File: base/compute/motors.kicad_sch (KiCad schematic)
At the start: 17 parts, among them U4 W25X20CLSN, U5 ICE40UP5K-SG48ITR-FPGA_Lattice

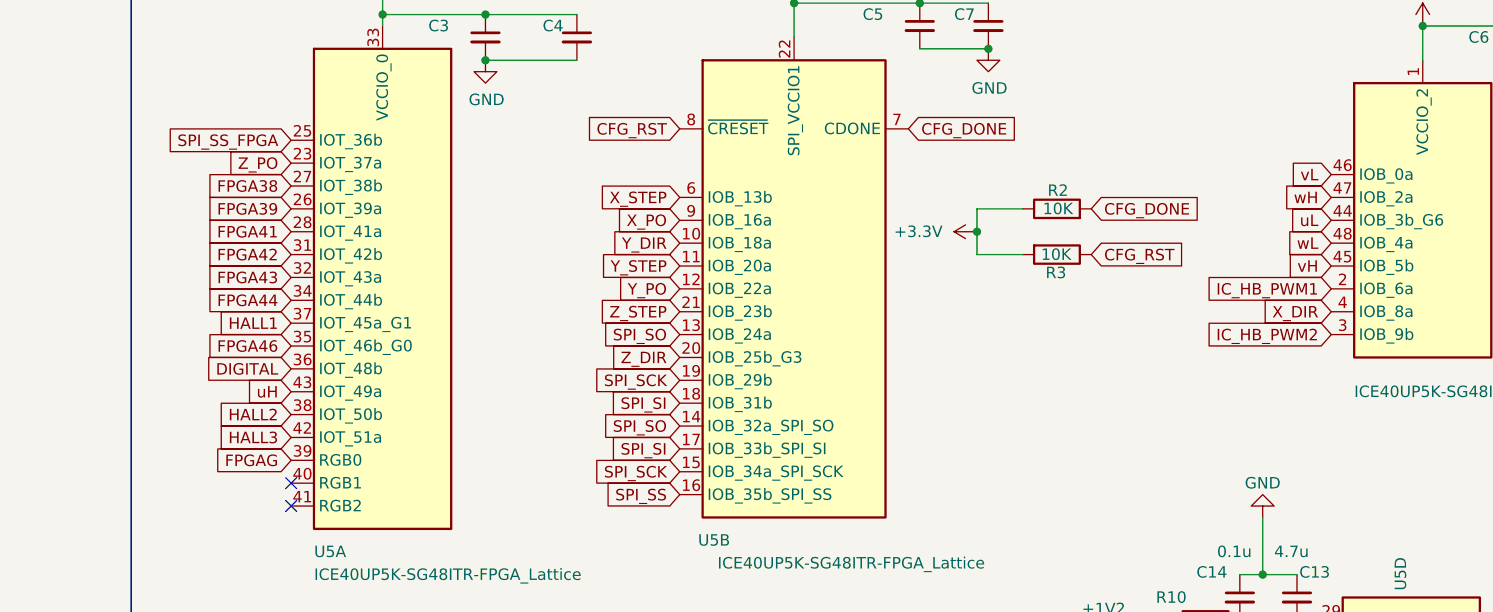
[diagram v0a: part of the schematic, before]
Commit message: retracking board
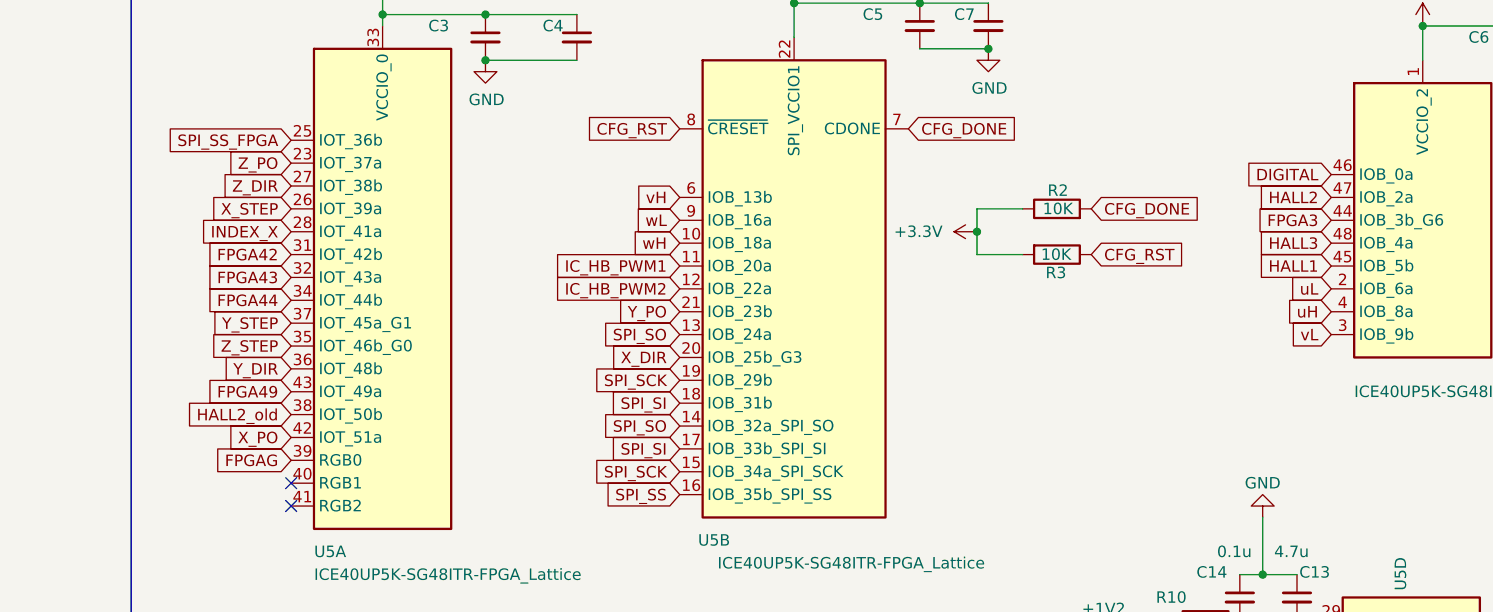
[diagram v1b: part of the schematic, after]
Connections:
- net FPGA38 is gone; now on net Z_DIR: U5.27 (IOT_38b)
- net FPGA39 is gone; now on net X_STEP: U5.26 (IOT_39a)
- net FPGA46 is gone; now on net Z_STEP: U5.35 (IOT_46b_G0)
- net DIGITAL: now also U5.46 (IOB_0a); no longer U5.36 (IOT_48b)
- net HALL1: now also U5.45 (IOB_5b); no longer U5.37 (IOT_45a_G1)
- net HALL2: now also U5.47 (IOB_2a); no longer U5.38 (IOT_50b)
- net HALL3: now also U5.48 (IOB_4a); no longer U5.42 (IOT_51a)
- net IC_HB_PWM1: now also U5.11 (IOB_20a); no longer U5.2 (IOB_6a)
- net IC_HB_PWM2: now also U5.12 (IOB_22a); no longer U5.3 (IOB_9b)
- net X_DIR: now also U5.20 (IOB_25b_G3); no longer U5.4 (IOB_8a)
- net X_PO: now also U5.42 (IOT_51a); no longer U5.9 (IOB_16a)
- net X_STEP: no longer U5.6 (IOB_13b)
- net Y_DIR: now also U5.36 (IOT_48b); no longer U5.10 (IOB_18a)
- net Y_PO: now also U5.21 (IOB_23b); no longer U5.12 (IOB_22a)
- net Y_STEP: now also U5.37 (IOT_45a_G1); no longer U5.11 (IOB_20a)
- net Z_DIR: no longer U5.20 (IOB_25b_G3)
- net Z_STEP: no longer U5.21 (IOB_23b)
- net uH: now also U5.4 (IOB_8a); no longer U5.43 (IOT_49a)
- net uL: now also U5.2 (IOB_6a); no longer U5.44 (IOB_3b_G6)
- net vH: now also U5.6 (IOB_13b); no longer U5.45 (IOB_5b)
- net vL: now also U5.3 (IOB_9b); no longer U5.46 (IOB_0a)
- net wH: now also U5.10 (IOB_18a); no longer U5.47 (IOB_2a)
- net wL: now also U5.9 (IOB_16a); no longer U5.48 (IOB_4a)
- net FPGA41 renamed INDEX_X
- new net FPGA3: U5.44 (IOB_3b_G6)
- new net FPGA49: U5.43 (IOT_49a)
- new net HALL2_old: U5.38 (IOT_50b)
